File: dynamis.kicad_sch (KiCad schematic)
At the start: 189 parts, among them J0 USB_C_Receptacle_USB2.0, SW00_00 SW_Push, SW00_01 SW_Push, SW00_02 SW_Push, SW00_03 SW_Push, SW00_04 SW_Push, SW00_05 SW_Push, SW00_06 SW_Push, SW01_00 SW_Push, SW01_01 SW_Push, SW01_02 SW_Push, SW01_03 SW_Push, SW01_04 SW_Push, SW01_05 SW_Push, SW01_06 SW_Push, SW02_01 SW_Push, SW02_02 SW_Push, SW02_03 SW_Push, SW02_04 SW_Push, SW02_05 SW_Push, SW02_06 SW_Push, SW03_00 SW_Push, SW03_02 SW_Push, SW03_03 SW_Push, SW03_04 SW_Push, SW03_05 SW_Push, SW03_06 SW_Push, SW04_00 SW_Push, SW04_01 SW_Push, SW04_02 SW_Push, SW04_03 SW_Push, SW04_05 SW_Push, SW04_06 SW_Push, SW05_01 SW_Push, SW05_02 SW_Push, SW05_03 SW_Push, SW05_04 SW_Push, SW05_05 SW_Push, SW05_06 SW_Push, SW06_00 SW_Push, SW06_01 SW_Push, SW06_02 SW_Push, SW06_03 SW_Push, SW06_04 SW_Push, SW06_05 SW_Push, SW06_06 SW_Push, SW07_01 SW_Push, SW07_02 SW_Push, SW07_03 SW_Push, SW07_04 SW_Push, SW07_05 SW_Push, SW07_06 SW_Push, SW08_00 SW_Push, SW08_02 SW_Push, SW08_03 SW_Push, SW08_04 SW_Push, SW08_05 SW_Push, SW08_06 SW_Push, SW09_00 SW_Push, SW09_01 SW_Push, SW09_02 SW_Push, SW09_03 SW_Push, SW09_04 SW_Push, SW09_05 SW_Push, SW09_06 SW_Push, U0 ATmega32U4-A, U1 PMW3360DM-T2QU, U2 TLV70019DDCR, U3 74LVC1T45GW,125, U4 74LVC1T45GW,125, U5 74LVC1T45GW,125, U6 74LVC1T45GW,125, U7 74LVC1T45GW,125, Y0 16Mhz

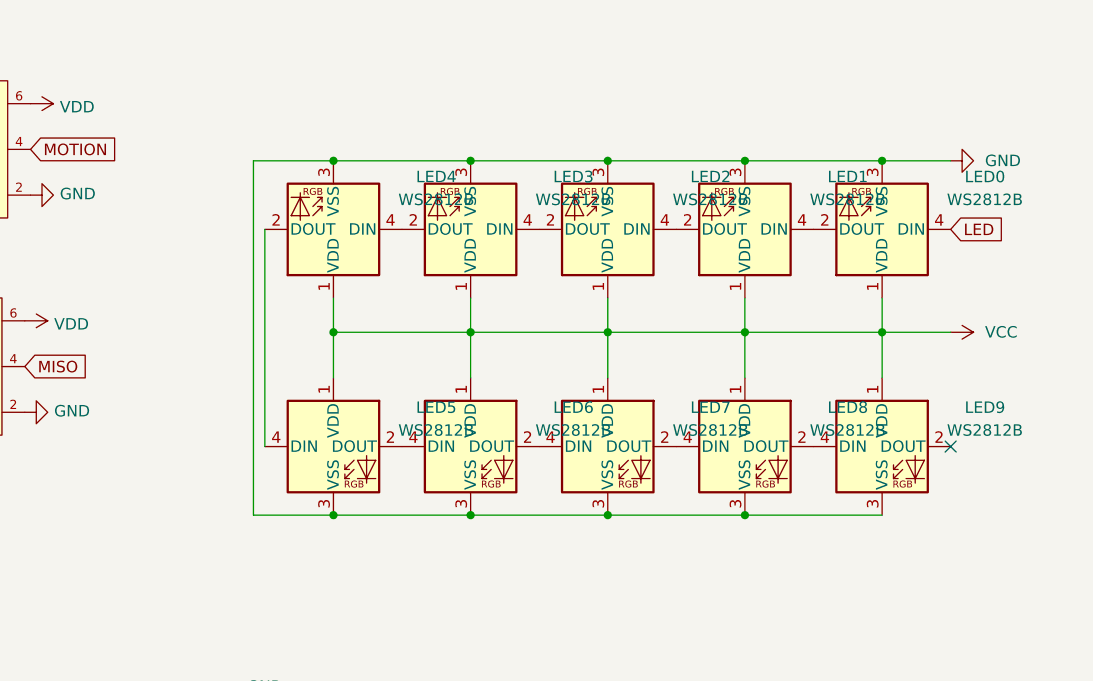
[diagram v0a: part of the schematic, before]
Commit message: wip
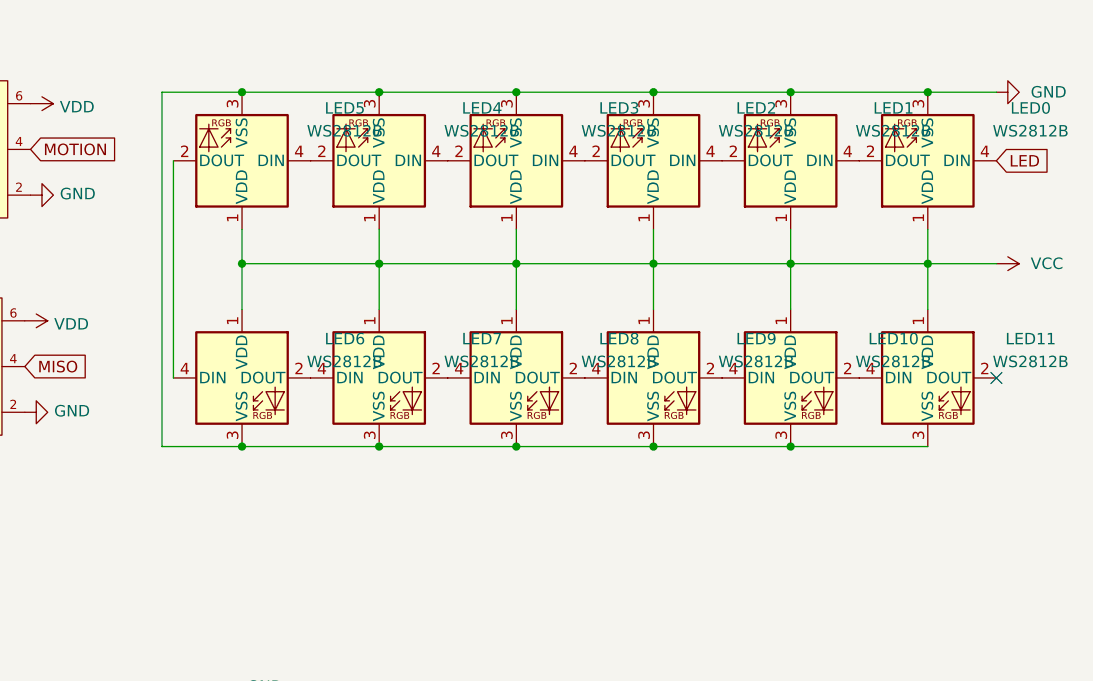
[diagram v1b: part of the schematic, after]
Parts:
- added LED5, LED6: WS2812B, LED_SMD:LED_WS2812B_PLCC4_5.0x5.0mm_P3.2mm, symbol LED:WS2812B
- renumbered LED8 to LED10, LED9 to LED11, LED5 to LED7, LED6 to LED8, LED7 to LED9
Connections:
- net GND: now also LED5.3 (VSS), LED6.3 (VSS)
- net VCC: now also LED5.1 (VDD), LED6.1 (VDD)
- net at LED7.4 (DIN): now also LED6.2 (DOUT); no longer LED4.2 (DOUT)
- new net: LED4.2 (DOUT), LED5.4 (DIN)
- new net: LED5.2 (DOUT), LED6.4 (DIN)
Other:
- moved on the sheet: LED0, LED1, LED10, LED11, LED2, LED3, LED4, LED7, LED8, LED9
